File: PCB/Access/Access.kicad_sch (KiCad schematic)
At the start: 63 parts, among them J1 USB-C, J2 RFID, J3 INPUTS, J4 USB-PROG, J5 POWER, J6 DOOR2, J7 DOOR1, J8 Shelly, Q2 PMF250XNEX, SW1 ESE13V01D, U1 MD8942, U10 ESP32-S3-MINI-1, U2 MD8942, U3 G3VM-41GR8, U8 G3VM-41GR8, U9 AA

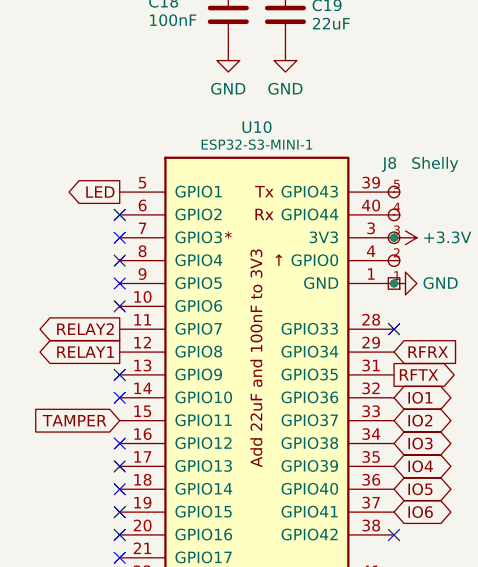
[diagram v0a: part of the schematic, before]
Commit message: Tweak
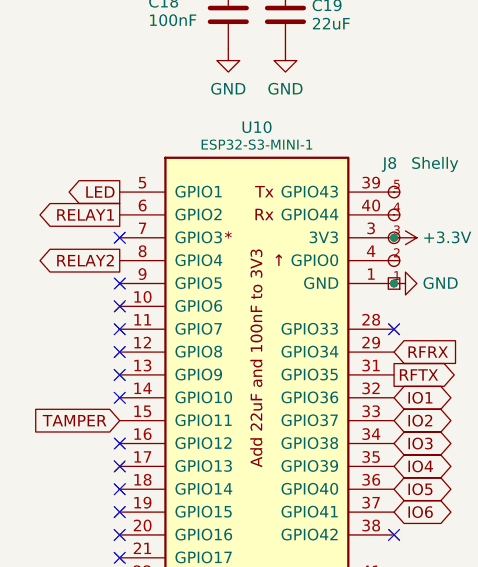
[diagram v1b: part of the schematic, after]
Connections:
- net RELAY1: now also U10.6 (GPIO2); no longer U10.12 (GPIO8)
- net RELAY2: now also U10.8 (GPIO4); no longer U10.11 (GPIO7)
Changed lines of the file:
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@@
   (no_connect (at 143.51 97.79))
   (no_connect (at 38.735 102.87))
-  (no_connect (at 38.735 57.15))
+  (no_connect (at 38.735 69.85))
   (no_connect (at 151.13 102.87))
   (no_connect (at 38.735 90.17))
@@
   (no_connect (at 38.735 95.25))
   (no_connect (at 38.735 87.63))
-  (no_connect (at 38.735 54.61))
-  (no_connect (at 38.735 59.69))
+  (no_connect (at 38.735 57.15))
+  (no_connect (at 38.735 67.31))
   (no_connect (at 158.75 97.79))
   (no_connect (at 205.74 37.465))
@@
     )
   )
-  (global_label "RELAY2" (shape output) (at 38.735 67.31 180) (fields_autoplaced)
-    (effects (font (size 1.27 1.27)) (justify right))
-    (property "Intersheetrefs" "${INTERSHEET_REFS}" (at 29.6496 67.31 0)
+  (global_label "RELAY2" (shape output) (at 38.735 59.69 180) (fields_autoplaced)
+    (effects (font (size 1.27 1.27)) (justify right))
+    (property "Intersheetrefs" "${INTERSHEET_REFS}" (at 29.6496 59.69 0)
       (effects (font (size 1.27 1.27)) (justify right) hide)
     )
@@
     )
   )
-  (global_label "RELAY1" (shape output) (at 38.735 69.85 180) (fields_autoplaced)
-    (effects (font (size 1.27 1.27)) (justify right))
-    (property "Intersheetrefs" "${INTERSHEET_REFS}" (at 29.577 69.7706 0)
-      (effects (font (size 1.27 1.27)) (justify right) hide)
-    )
+  (global_label "RELAY1" (shape output) (at 38.735 54.61 180) (fields_autoplaced)
+    (effects (font (size 1.27 1.27)) (justify right))
+    (property "Intersheetrefs" "${INTERSHEET_REFS}" (at 29.577 54.5306 0)
+      (effects (font (size 1.27 1.27)) (justify right) hide)
+    )
